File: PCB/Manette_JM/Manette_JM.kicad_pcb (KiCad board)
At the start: 4 copper layers, 110 x 60 mm, 43 parts, among them J1 Jack 1, J10 Jack 10, J11 Jack 11, J12 Jack 12, J13 Jack 13, J14 Jack 14, J15 Bouton 1, J16 Bouton 2, J17 Bouton 3, J18 Bouton 4, J19 Bouton 5, J2 Jack 2, J20 DEL PWR, J21 Joystick 0, J3 Jack 3, J4 Jack 4, J5 Jack 5, J6 Jack 6, J7 Jack 7, J8 Jack 8, J9 Jack 9, U1 NodeMCU1.0(ESP-12E), U2 ProMicro

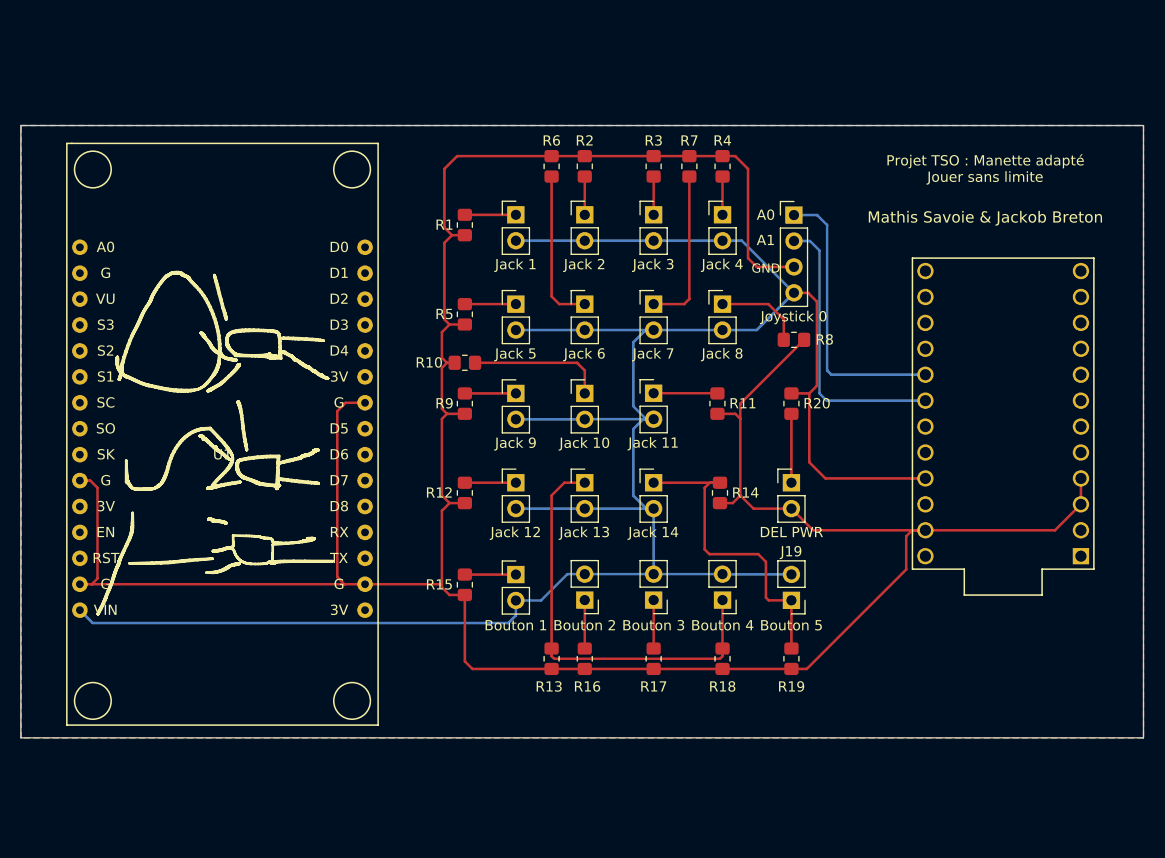
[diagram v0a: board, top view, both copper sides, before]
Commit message: quick chanfes
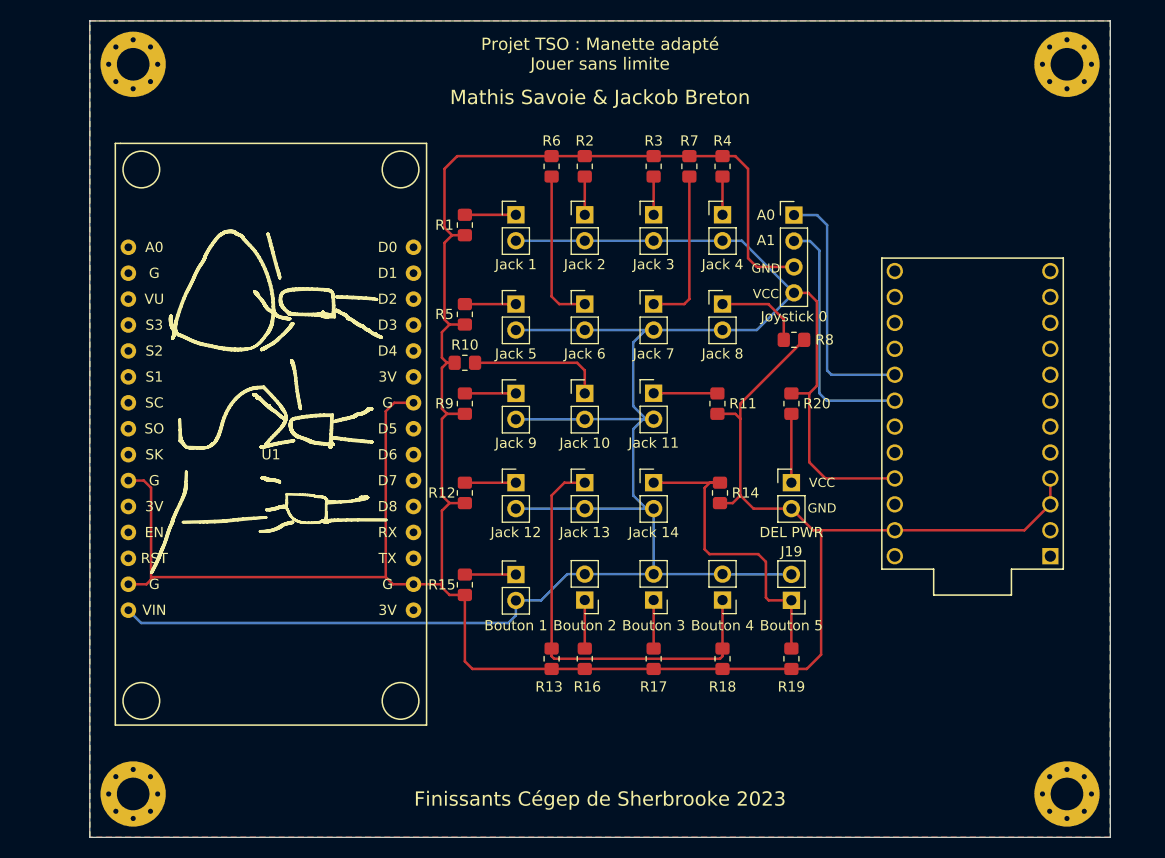
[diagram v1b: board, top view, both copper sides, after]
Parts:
- added H1: MountingHole_Pad, MountingHole:MountingHole_3.2mm_M3_Pad_Via, F.Cu at (105.8, 39.8)
- added H2: MountingHole_Pad, MountingHole:MountingHole_3.2mm_M3_Pad_Via, F.Cu at (105.8, 111.2)
- added H3: MountingHole_Pad, MountingHole:MountingHole_3.2mm_M3_Pad_Via, F.Cu at (197.2, 111.2)
- added H4: MountingHole_Pad, MountingHole:MountingHole_3.2mm_M3_Pad_Via, F.Cu at (197.2, 39.8)
- moved U1 4.75 mm to (119.2, 78.0)
- moved U2 3.00 mm to (188.0, 74.0)
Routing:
- net GND: track 285.2 -> 271.9 mm
- net Net-(U1-Pad18): track 102.8 -> 92.6 mm
- net Net-(U1-Pad19): track 98.8 -> 90.9 mm
- net VCC: track 219.8 -> 212.1 mm
- net D2: track 96.7 -> 92.7 mm
- net D3: track 83.6 -> 80.0 mm
- net D4: track 72.2 -> 68.6 mm
- net D5: track 60.4 -> 57.2 mm
- net D16: track 83.8 -> 80.6 mm
- net D10: track 54.5 -> 51.3 mm
- net D9: track 45.5 -> 42.5 mm
- net D8: track 64.0 -> 61.0 mm
- net D7: track 70.7 -> 67.7 mm
- net D6: track 68.5 -> 65.5 mm
- net D20: track 75.5 -> 72.5 mm
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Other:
- board size 110 x 60 mm -> 100 x 80 mm
- board text added: "Finissants Cégep de Sherbrooke 2023"
- board text added: "VCC"
